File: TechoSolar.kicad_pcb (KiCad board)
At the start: 2 copper layers, 81.5 x 46.8 mm, 41 parts, among them J1 Conn_02x04_Odd_Even, J2 DE9_Pins, J3 Conn_PIC_ICSP_ICD, J7 Conn_01x02, J8 Conn_01x02, J9 Conn_01x02, SW1 SW_Push, SW2 SW_DIP_x01, SW3 MPB01-1B33-S-D, SW4 MPB01-1B33-S-D, U1 PIC18F2580-I_ML, U2 L293DD, U3 TCAN332D, U4 LT1117CST-3.3, Y1 Crystal

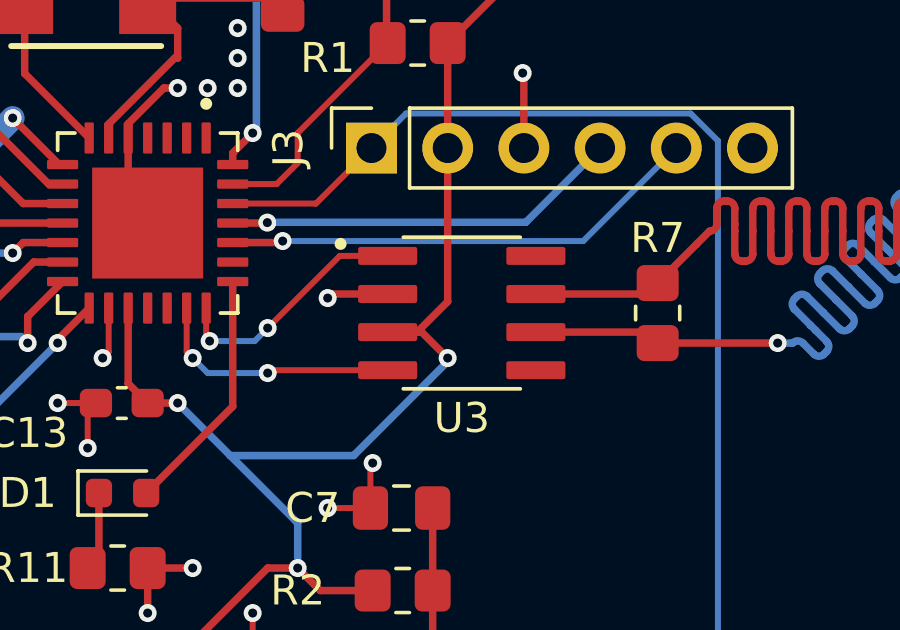
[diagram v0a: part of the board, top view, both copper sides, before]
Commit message: Update TechoSolar.kicad_pcb
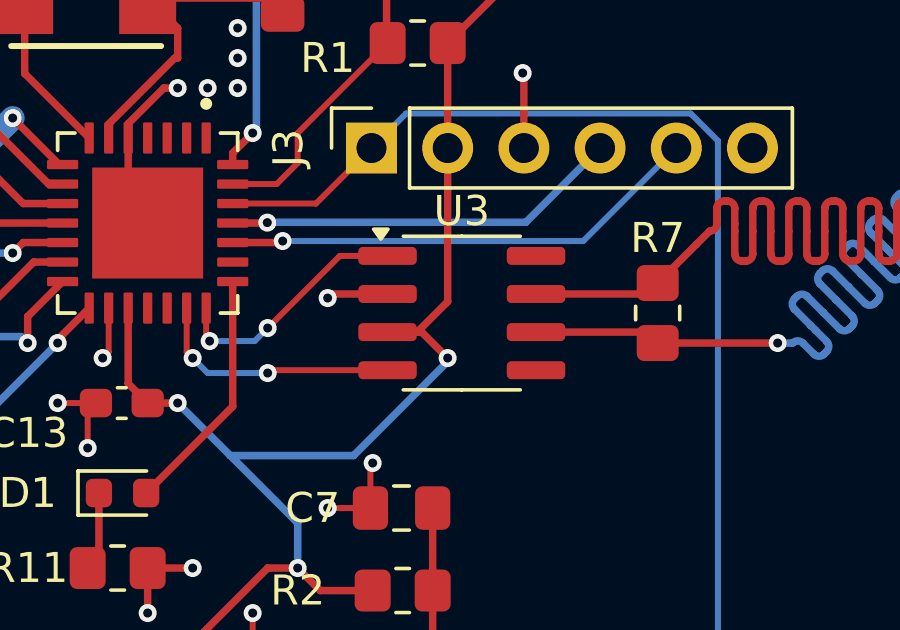
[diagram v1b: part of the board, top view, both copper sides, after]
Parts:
- U3: footprint User_Library:SOIC127P599X175-8N -> Package_SO:SOIC-8_3.9x4.9mm_P1.27mm
